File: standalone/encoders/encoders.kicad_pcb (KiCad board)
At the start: 2 copper layers, 78.5 x 35.6 mm, 20 parts, among them SW1 RotaryEncoder_Switch, SW2 RotaryEncoder_Switch, SW3 RotaryEncoder_Switch, SW4 RotaryEncoder_Switch, SW5 SW_SPDT, SW6 SW_Push, U1 ProMicro

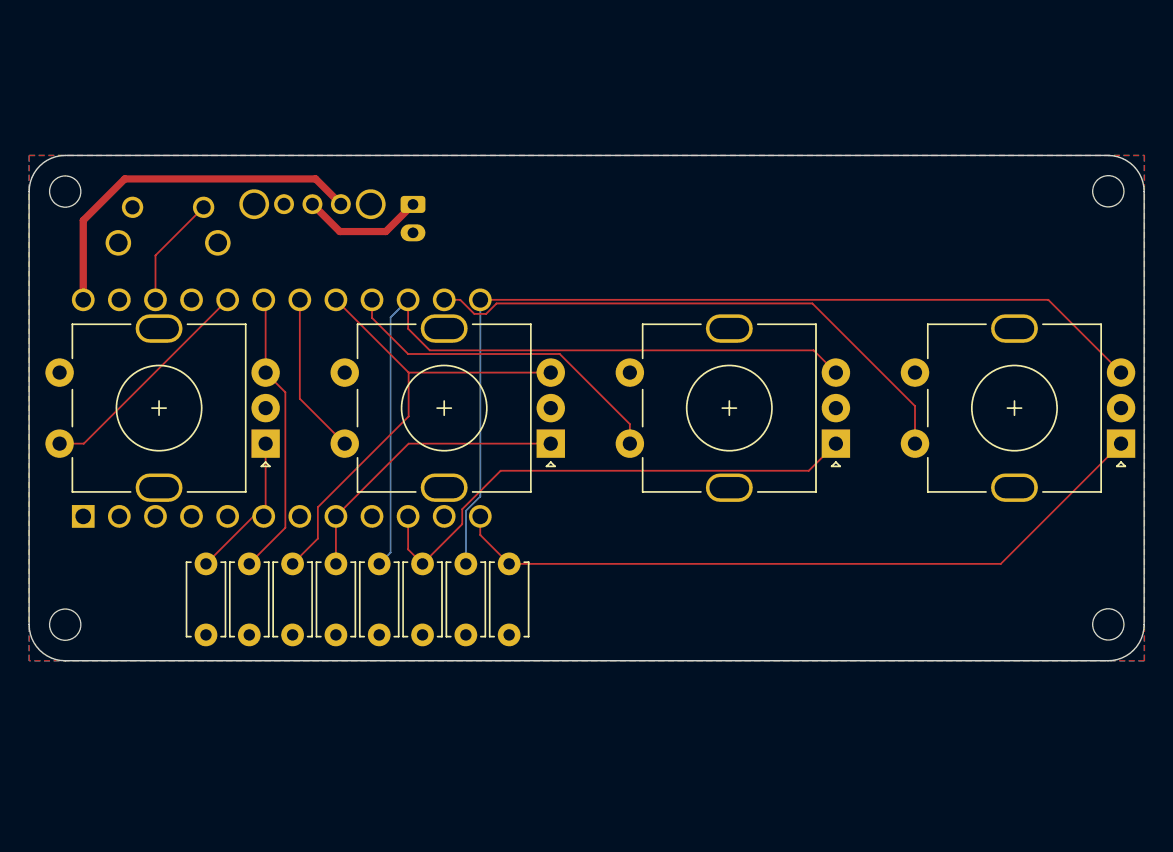
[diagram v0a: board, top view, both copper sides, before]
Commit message: add ocelots
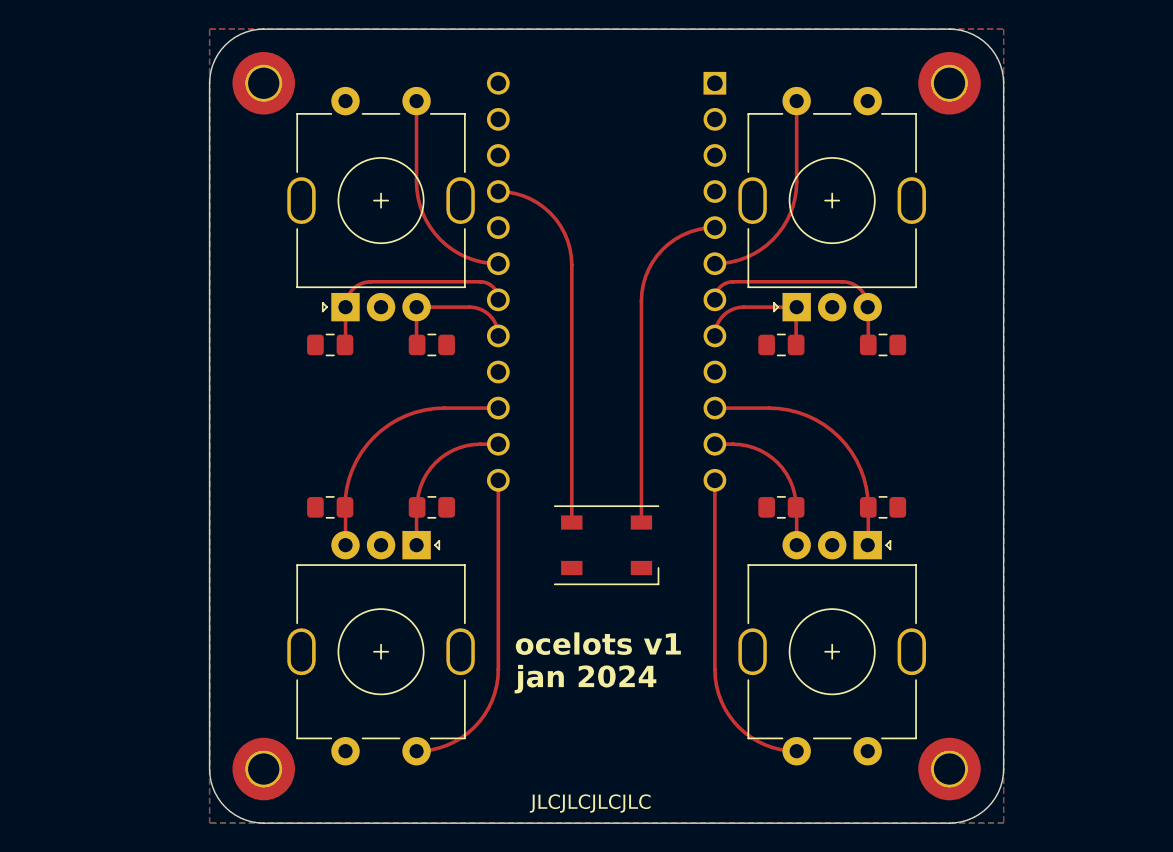
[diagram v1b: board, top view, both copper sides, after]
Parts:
- removed BT1: Battery_Cell, Connector_JST:JST_PH_S2B-PH-K_1x02_P2.00mm_Horizontal
- removed SW5: SW_SPDT, Pale Slim Ghost:EG1247
- removed SW6: SW_Push, Pale Slim Ghost:MJPT1117 Tactile Switch
- added D2: SK6812, LED_SMD:LED_SK6812_PLCC4_5.0x5.0mm_P3.2mm, F.Cu at (170.2, 73.2)
- C1, C2, C3, C4, C5, C6, C7, C8: footprint Capacitor_THT:C_Disc_D5.0mm_W2.5mm_P5.00mm -> Capacitor_SMD:C_0805_2012Metric_Pad1.18x1.45mm_HandSolder
- H1, H2, H3, H4: footprint MountingHole:MountingHole_2.2mm_M2 -> MountingHole:MountingHole_2.2mm_M2_Pad_TopOnly
- U1: moved to B.Cu
- moved C4 44.3 mm to (189.6, 59.1), turned to 0 degrees
- moved C3 37.4 mm to (182.5, 59.1), turned to 0 degrees
- moved SW2 31.0 mm to (186.1, 48.9), turned to 90 degrees
- moved SW3 29.9 mm to (154.3, 80.6), turned to -90 degrees
- moved C7 27.8 mm to (189.6, 70.5), turned to 180 degrees
- moved U1 24.5 mm to (170.2, 54.6), turned to -90 degrees
- moved C8 22.6 mm to (182.5, 70.5), turned to 180 degrees
- moved C1 22.2 mm to (150.7, 59.1), turned to 0 degrees
- moved SW4 21.4 mm to (186.1, 80.6), turned to -90 degrees
- moved SW1 21.4 mm to (154.3, 48.9), turned to 90 degrees
- moved C2 20.1 mm to (157.9, 59.1), turned to 0 degrees
- moved H3 17.3 mm to (146.1, 88.9)
- moved H1 15.9 mm to (146.1, 40.6)
- moved H4 15.1 mm to (194.3, 88.9)
- moved H2 13.5 mm to (194.3, 40.6)
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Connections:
- SW1 pad S1: GND -> Encoder 1 Switch
- SW1 pad S2: Encoder 1 Switch -> GND
- SW4 pad S1: GND -> Encoder 4 Switch
- SW4 pad S2: Encoder 4 Switch -> GND
- U1 pad 10: Encoder 3 A -> Encoder 4 A
- U1 pad 11: unconnected-(U1-Pad11) -> Encoder 4 B
- U1 pad 12: Encoder 4 A -> Encoder 4 Switch
- U1 pad 13: Encoder 4 B -> Encoder 3 Switch
- U1 pad 14: Encoder 4 Switch -> Encoder 3 A
- U1 pad 16: Encoder 3 Switch -> unconnected-(U1-B1/15-Pad16)
- U1 pad 17: Encoder 2 B -> Encoder 1 B
- U1 pad 18: Encoder 2 Switch -> Encoder 1 A
- U1 pad 19: Encoder 1 B -> Encoder 1 Switch
- U1 pad 20: Encoder 1 Switch -> unconnected-(U1-F4/A3-Pad20)
- U1 pad 21: +5V -> +3.3V
- U1 pad 5: unconnected-(U1-Pad5) -> LED
- U1 pad 6: Encoder 1 A -> Encoder 2 Switch
- U1 pad 7: unconnected-(U1-Pad7) -> Encoder 2 B
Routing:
- net Encoder 4 B: track 66.2 -> 10.9 mm
- net Encoder 3 B: track 52.8 -> 17.4 mm
- net Encoder 4 A: track 50.7 -> 17.4 mm
- net Encoder 3 A: track 37.0 -> 10.9 mm
- net +3.3V: track 0.00 -> 26.0 mm
- net +BATT: track 25.7 -> 0.00 mm
- net LED: track 0.00 -> 23.5 mm
- net Encoder 2 B: track 34.1 -> 15.1 mm
- net Encoder 4 Switch: track 39.5 -> 22.1 mm
- net Encoder 2 A: track 20.6 -> 9.51 mm
- net Encoder 1 B: track 20.3 -> 9.51 mm
- net Net-(BT1-Pad1): track 8.66 -> 0.00 mm
- net Reset: track 7.91 -> 0.00 mm
- net Encoder 1 A: track 10.6 -> 15.1 mm
- net Encoder 2 Switch: track 11.4 -> 14.5 mm
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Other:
- board size 78.5 x 35.6 mm -> 55.9 x 55.9 mm
- board text added: "JLCJLCJLCJLC"
- board text added: "jan 2024"
- board text added: "ocelots v1"
